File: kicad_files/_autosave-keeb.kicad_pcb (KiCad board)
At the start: 2 copper layers, 369.3 x 148.8 mm, 232 parts, among them SW10 SW_Push, SW11 SW_Push, SW12 SW_Push, SW13 SW_Push, SW14 SW_Push, SW15 SW_Push, SW16 SW_Push, SW17 SW_Push, SW18 SW_Push, SW19 SW_Push, SW2 RotaryEncoder_Switch, SW20 SW_Push, SW21 SW_Push, SW22 SW_Push, SW23 SW_Push, SW24 SW_Push, SW25 SW_Push, SW26 SW_Push, SW27 SW_Push, SW28 SW_Push, SW29 SW_Push, SW3 SW_Push, SW30 SW_Push, SW31 SW_Push, SW32 SW_Push, SW33 SW_Push, SW34 SW_Push, SW35 SW_Push, SW36 SW_Push, SW37 SW_Push, SW38 SW_Push, SW39 SW_Push, SW4 SW_Push, SW40 SW_Push, SW41 SW_Push, SW42 SW_Push, SW43 SW_Push, SW44 SW_Push, SW45 SW_Push, SW46 SW_Push, SW47 SW_Push, SW48 SW_Push, SW49 SW_Push, SW5 SW_Push, SW50 SW_Push, SW51 SW_Push, SW52 SW_Push, SW53 SW_Push, SW54 SW_Push, SW55 SW_Push, SW56 SW_Push, SW6 SW_Push, SW7 SW_Push, SW8 SW_Push, SW9 SW_Push, U2 ER_OLEDM0.91_1x-I2C

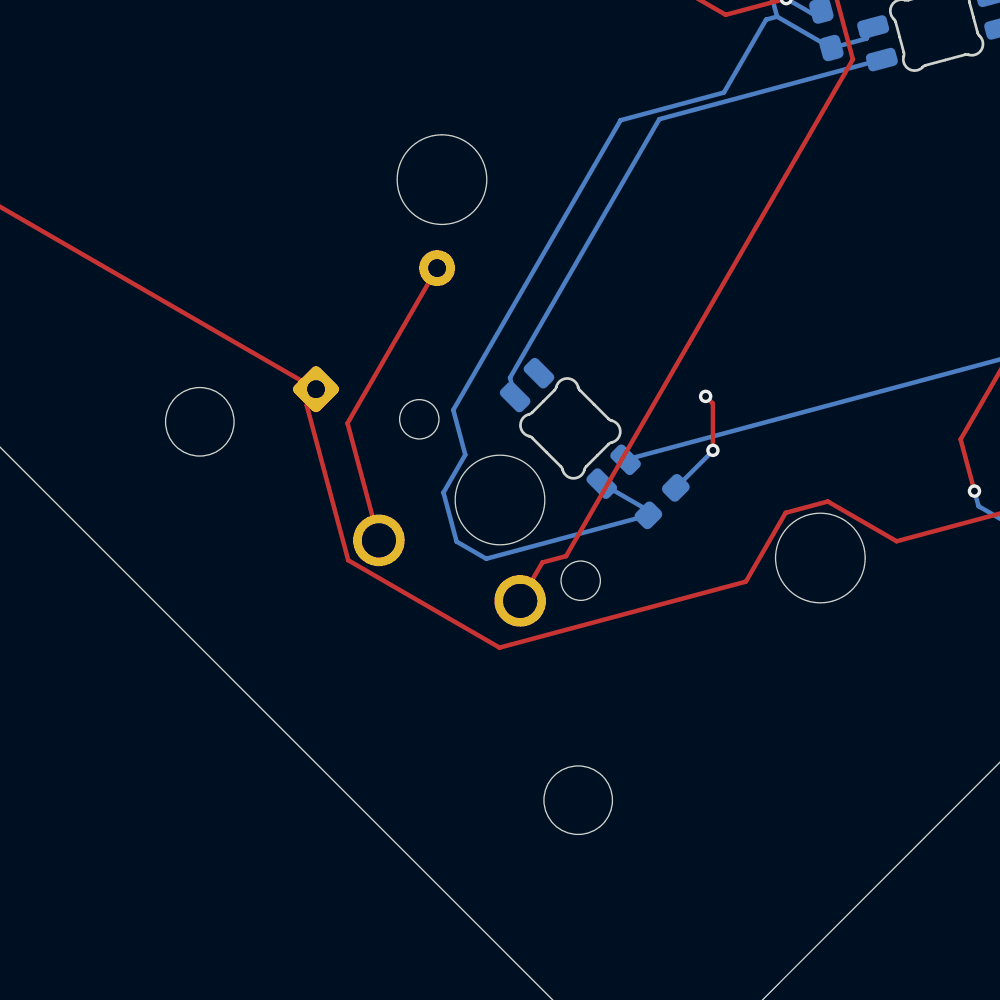
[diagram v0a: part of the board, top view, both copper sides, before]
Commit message: Case done (!!!)
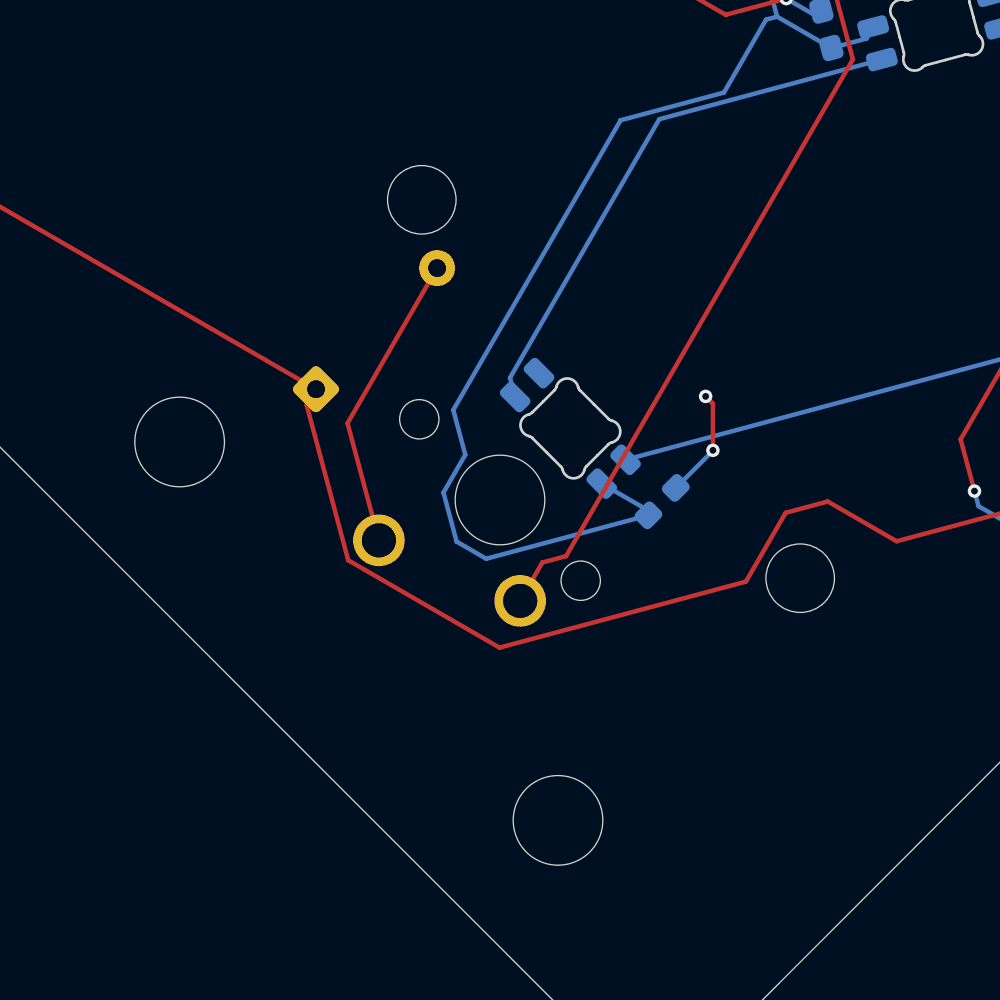
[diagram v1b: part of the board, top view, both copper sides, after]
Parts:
- turned S1 to -45 degrees
